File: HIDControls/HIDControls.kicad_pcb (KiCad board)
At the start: 2 copper layers, 83.8 x 91.4 mm, 70 parts, among them M1 ModulePlug, M10 ModulePlug, M11 ModulePlug, M12 ModulePlug, M2 ModulePlug, M3 ModulePlug, M4 ModulePlug, M5 ModulePlug, M6 ModulePlug, M7 ModulePlug, M8 ModulePlug, M9 ModulePlug, SW1 6mm, SW10 6mm, SW11 6mm, SW12 6mm, SW13 6mm, SW14 6mm, SW2 6mm, SW3 ALPS EC11, SW4 SS12D10, SW5 ALPS EC11, SW6 8x8 SWITCH, SW7 5mm TOGGLE, SW8 6mm, SW9 6mm

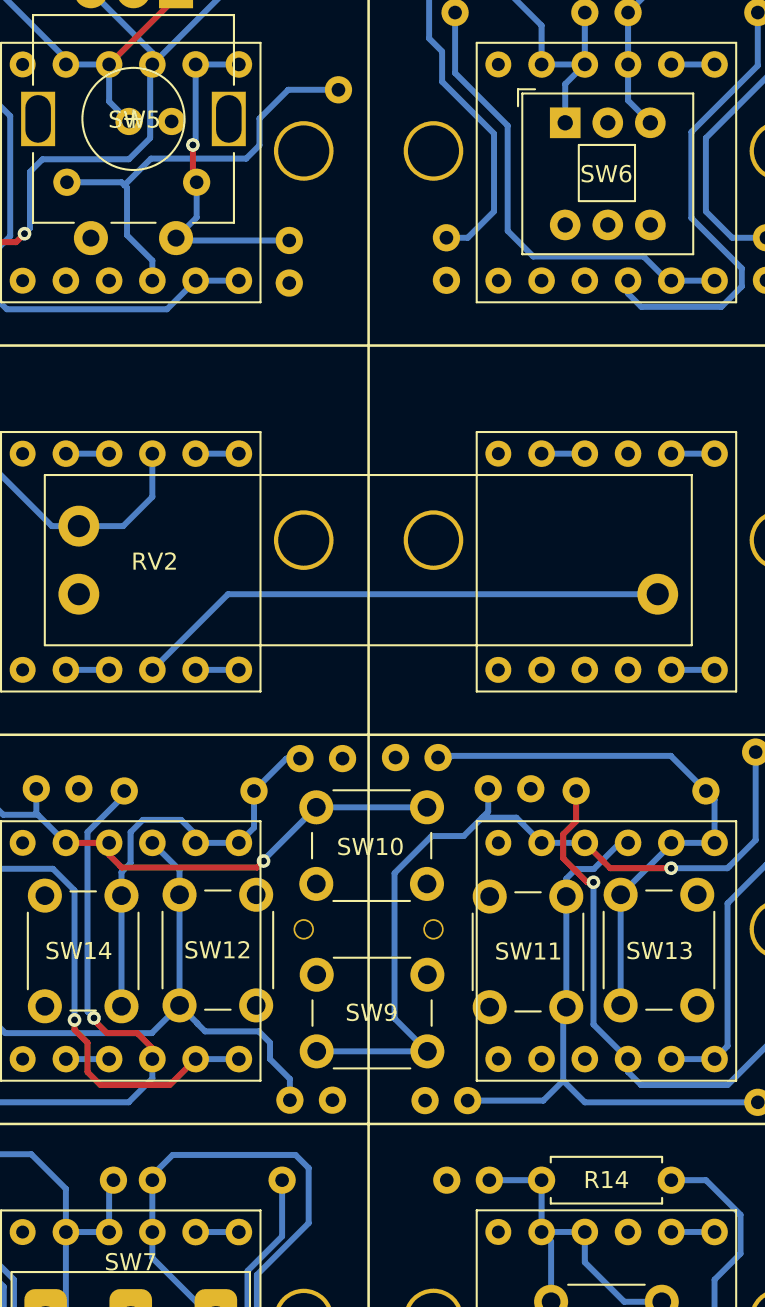
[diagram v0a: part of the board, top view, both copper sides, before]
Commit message: Minor layout tweaks
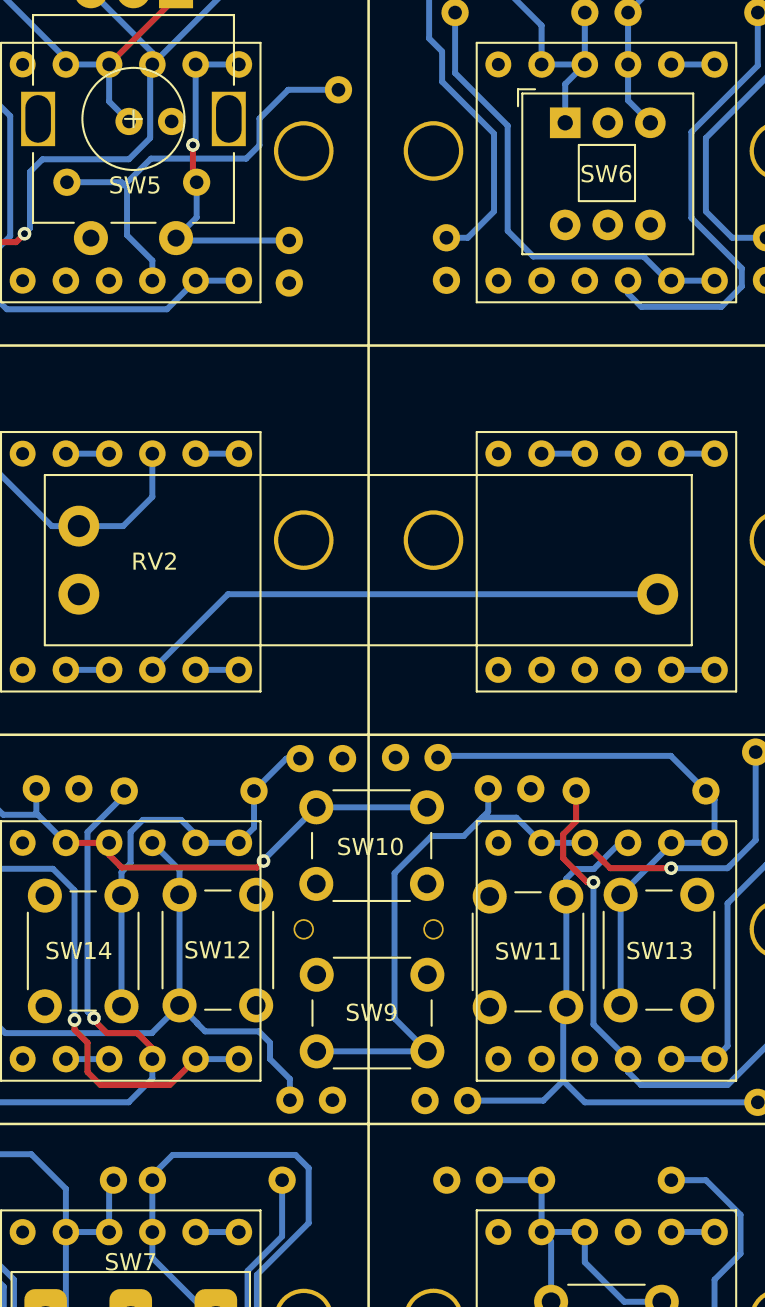
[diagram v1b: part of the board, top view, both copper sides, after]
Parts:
- R14: moved to B.Cu
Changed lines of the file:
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@@
     (property "Sheetname" "")
     (attr through_hole)
-    (fp_text reference "SW5" (at 7.55 2.44 180) (layer "F.SilkS")
+    (fp_text reference "SW5" (at 11.412 2.406) (layer "F.SilkS")
       (effects (font (size 1 1) (thickness 0.15)))
     )
@@
     )
   )
-  (footprint "Resistor_THT:R_Axial_DIN0207_L6.3mm_D2.5mm_P7.62mm_Horizontal" (layer "F.Cu")
-    (at 154.94 125.222)
-    (descr "Resistor, Axial_DIN0207 series, Axial, Horizontal, pin pitch=7.62mm, 0.25W = 1/4W, length*diameter=6.3*2.5mm^2, http://cdn-reichelt.de/documents/datenblatt/B400/1_4W%23YAG.pdf")
-    (tags "Resistor Axial_DIN0207 series Axial Horizontal pin pitch 7.62mm 0.25W = 1/4W length 6.3mm diameter 2.5mm")
-    (property "Sheetfile" "HIDControls.kicad_sch")
-    (property "Sheetname" "")
-    (attr through_hole)
-    (fp_text reference "R14" (at 3.81 0) (layer "F.SilkS")
-      (effects (font (size 1 1) (thickness 0.15)))
-    )
-    (fp_text value "10k" (at 3.81 2.37) (layer "F.Fab")
-      (effects (font (size 1 1) (thickness 0.15)))
-    )
-    (fp_text user "${REFERENCE}" (at 3.81 0) (layer "F.Fab")
-      (effects (font (size 1 1) (thickness 0.15)))
-    )
-    (fp_line (start 0.54 1.37) (end 7.08 1.37) (layer "F.SilkS") (width 0.12))
-    (fp_line (start 0.54 -1.04) (end 0.54 -1.37) (layer "F.SilkS") (width 0.12))
-    (fp_line (start 0.54 1.04) (end 0.54 1.37) (layer "F.SilkS") (width 0.12))
-    (fp_line (start 0.54 -1.37) (end 7.08 -1.37) (layer "F.SilkS") (width 0.12))
-    (fp_line (start 7.08 -1.37) (end 7.08 -1.04) (layer "F.SilkS") (width 0.12))
-    (fp_line (start 7.08 1.37) (end 7.08 1.04) (layer "F.SilkS") (width 0.12))
-    (fp_line (start -1.05 1.5) (end 8.67 1.5) (layer "F.CrtYd") (width 0.05))
-    (fp_line (start -1.05 -1.5) (end -1.05 1.5) (layer "F.CrtYd") (width 0.05))
-    (fp_line (start 8.67 -1.5) (end -1.05 -1.5) (layer "F.CrtYd") (width 0.05))
-    (fp_line (start 8.67 1.5) (end 8.67 -1.5) (layer "F.CrtYd") (width 0.05))
-    (fp_line (start 0.66 -1.25) (end 0.66 1.25) (layer "F.Fab") (width 0.1))
-    (fp_line (start 6.96 -1.25) (end 0.66 -1.25) (layer "F.Fab") (width 0.1))
-    (fp_line (start 6.96 1.25) (end 6.96 -1.25) (layer "F.Fab") (width 0.1))
-    (fp_line (start 0 0) (end 0.66 0) (layer "F.Fab") (width 0.1))
-    (fp_line (start 7.62 0) (end 6.96 0) (layer "F.Fab") (width 0.1))
-    (fp_line (start 0.66 1.25) (end 6.96 1.25) (layer "F.Fab") (width 0.1))
-    (pad "1" thru_hole circle (at 0 0) (size 1.6 1.6) (drill 0.8) (layers *.Cu *.Mask)
-      (net 70 "Net-(M11-Pad4)") (pintype "passive"))
-    (pad "2" thru_hole oval (at 7.62 0) (size 1.6 1.6) (drill 0.8) (layers *.Cu *.Mask)
-      (net 69 "Net-(M11-Pad3)") (pintype "passive"))
-    (model "${KICAD6_3DMODEL_DIR}/Resistor_THT.3dshapes/R_Axial_DIN0207_L6.3mm_D2.5mm_P7.62mm_Horizontal.wrl"
-      (offset (xyz 0 0 0))
-      (scale (xyz 1 1 1))
-      (rotate (xyz 0 0 0))
-    )
-  )
   (footprint "HIDControls:ModulePlug" (layer "F.Cu")
     (at 130.81 87.63)
@@
     (model "${KICAD6_3DMODEL_DIR}/Resistor_THT.3dshapes/R_Axial_DIN0207_L6.3mm_D2.5mm_P7.62mm_Horizontal.wrl"
       (offset (xyz 0 0 0))
+      (scale (xyz 1 1 1))
+      (rotate (xyz 0 0 0))
+    )
+  )
+  (footprint "Resistor_THT:R_Axial_DIN0207_L6.3mm_D2.5mm_P7.62mm_Horizontal" (layer "B.Cu")
+    (at 154.94 125.222)
+    (descr "Resistor, Axial_DIN0207 series, Axial, Horizontal, pin pitch=7.62mm, 0.25W = 1/4W, length*diameter=6.3*2.5mm^2, http://cdn-reichelt.de/documents/datenblatt/B400/1_4W%23YAG.pdf")
+    (tags "Resistor Axial_DIN0207 series Axial Horizontal pin pitch 7.62mm 0.25W = 1/4W length 6.3mm diameter 2.5mm")
+    (property "Sheetfile" "HIDControls.kicad_sch")
+    (property "Sheetname" "")
+    (attr through_hole)
+    (fp_text reference "R14" (at 3.81 0) (layer "B.SilkS")
+      (effects (font (size 1 1) (thickness 0.15)) (justify mirror))
+    )
+    (fp_text value "10k" (at 3.81 -2.37) (layer "B.Fab")
+      (effects (font (size 1 1) (thickness 0.15)) (justify mirror))
+    )
+    (fp_text user "${REFERENCE}" (at 3.81 0) (layer "B.Fab")
+      (effects (font (size 1 1) (thickness 0.15)) (justify mirror))
+    )
+    (fp_line (start 0.54 -1.37) (end 7.08 -1.37) (layer "B.SilkS") (width 0.12))
+    (fp_line (start 0.54 1.04) (end 0.54 1.37) (layer "B.SilkS") (width 0.12))
+    (fp_line (start 0.54 -1.04) (end 0.54 -1.37) (layer "B.SilkS") (width 0.12))
+    (fp_line (start 0.54 1.37) (end 7.08 1.37) (layer "B.SilkS") (width 0.12))
+    (fp_line (start 7.08 1.37) (end 7.08 1.04) (layer "B.SilkS") (width 0.12))
+    (fp_line (start 7.08 -1.37) (end 7.08 -1.04) (layer "B.SilkS") (width 0.12))
+    (fp_line (start -1.05 -1.5) (end 8.67 -1.5) (layer "B.CrtYd") (width 0.05))
+    (fp_line (start -1.05 1.5) (end -1.05 -1.5) (layer "B.CrtYd") (width 0.05))
+    (fp_line (start 8.67 1.5) (end -1.05 1.5) (layer "B.CrtYd") (width 0.05))
+    (fp_line (start 8.67 -1.5) (end 8.67 1.5) (layer "B.CrtYd") (width 0.05))
+    (fp_line (start 0.66 1.25) (end 0.66 -1.25) (layer "B.Fab") (width 0.1))
+    (fp_line (start 6.96 1.25) (end 0.66 1.25) (layer "B.Fab") (width 0.1))
+    (fp_line (start 6.96 -1.25) (end 6.96 1.25) (layer "B.Fab") (width 0.1))
+    (fp_line (start 0 0) (end 0.66 0) (layer "B.Fab") (width 0.1))
+    (fp_line (start 7.62 0) (end 6.96 0) (layer "B.Fab") (width 0.1))
+    (fp_line (start 0.66 -1.25) (end 6.96 -1.25) (layer "B.Fab") (width 0.1))
+    (pad "1" thru_hole circle (at 0 0) (size 1.6 1.6) (drill 0.8) (layers *.Cu *.Mask)
+      (net 70 "Net-(M11-Pad4)") (pintype "passive"))
+    (pad "2" thru_hole oval (at 7.62 0) (size 1.6 1.6) (drill 0.8) (layers *.Cu *.Mask)
+      (net 69 "Net-(M11-Pad3)") (pintype "passive"))
+    (model "${KICAD6_3DMODEL_DIR}/Resistor_THT.3dshapes/R_Axial_DIN0207_L6.3mm_D2.5mm_P7.62mm_Horizontal.wrl"
+      (offset (xyz 0 0 0))
